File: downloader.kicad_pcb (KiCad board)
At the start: 2 copper layers, 30 x 15 mm, 16 parts, among them J1 USB_C_Receptacle_USB2.0, J2 Conn_01x06_Female, Q1 SS8050-G, Q2 SS8050-G, SW1 SW_Push, SW2 SW_Push, U1 AMS1117-3.3, U2 ch340k

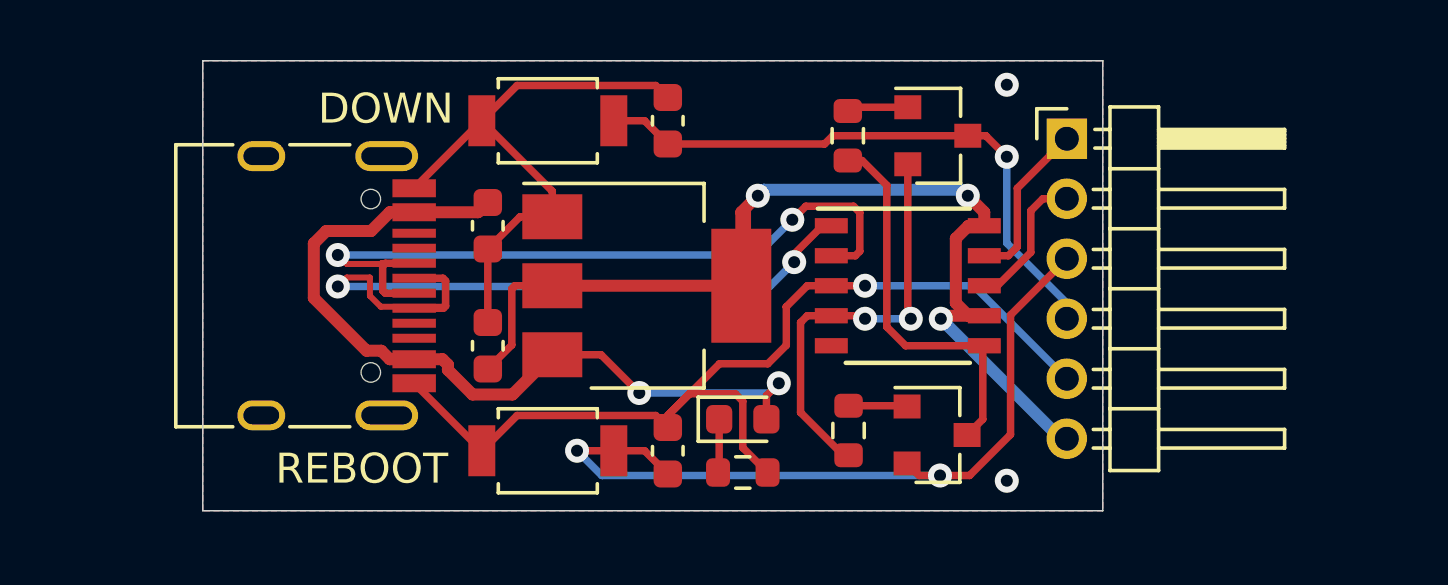
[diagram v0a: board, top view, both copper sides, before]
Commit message: version2.0
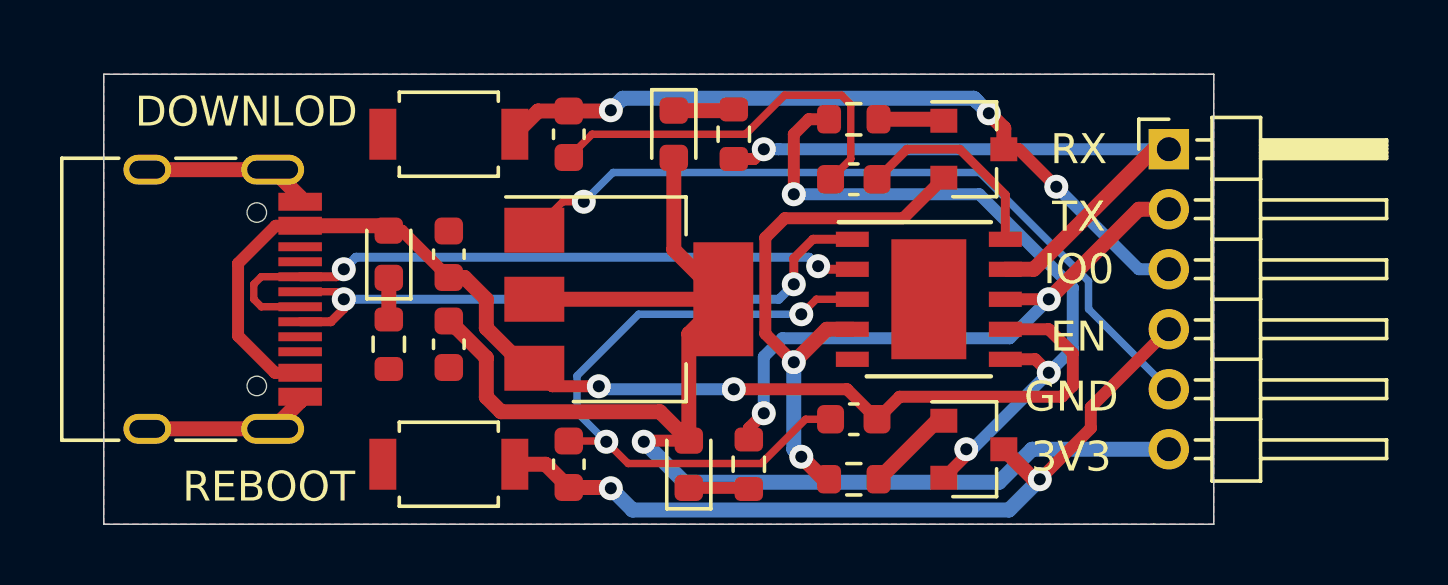
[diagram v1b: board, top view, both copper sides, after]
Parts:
- added C5: 0.1uf, Capacitor_SMD:C_0603_1608Metric, F.Cu at (112.2, 87.5)
- added C6: 0.1uf, Capacitor_SMD:C_0603_1608Metric, F.Cu at (112.2, 98.5)
- added D2: LED, Diode_SMD:D_0603_1608Metric, F.Cu at (115.7, 87.5)
- added D3: LED, Diode_SMD:D_0603_1608Metric, F.Cu at (116.2, 98.5)
- added R4: 10k, Resistor_SMD:R_0603_1608Metric, F.Cu at (121.7, 99.0)
- added R5: 10k, Resistor_SMD:R_0603_1608Metric, F.Cu at (121.7, 87.0)
- C2: value 0.1uf -> 10uf
- C3: value 10uf -> 0.1uf
- C4: value 0.1uf -> 0.1UF
- R1: value 470 -> 10k
- U2: footprint Package_SO:SSOP-10_3.9x4.9mm_P1.00mm -> my:ESSOP-10_3.9x4.9mm_P1.00mm
- moved C3 13.4 mm to (121.7, 89.0), turned to 0 degrees
- moved D1 13.0 mm to (106.2, 91.5), turned to 90 degrees
- moved R1 12.6 mm to (106.2, 94.5), turned to 270 degrees
- moved C2 10.4 mm to (108.2, 94.5), turned to 270 degrees
- moved C4 6.29 mm to (121.7, 97.0), turned to 0 degrees
- moved J1 3.83 mm to (99.2, 93.0)
- moved R2 3.80 mm to (117.7, 87.5)
- moved R3 3.51 mm to (118.2, 98.5), turned to 90 degrees
- moved J2 3.42 mm to (132.2, 88.0)
- moved SW1 3.33 mm to (108.2, 87.5)
- moved SW2 3.33 mm to (108.2, 98.5)
- moved C1 1.61 mm to (108.2, 91.5), turned to 90 degrees
- moved Q2 1.31 mm to (125.7, 98.0)
- moved Q1 1.28 mm to (125.7, 88.0)
- moved U2 0.83 mm to (124.2, 93.0)
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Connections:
- C1 pad 1: Net-(C1-Pad1) -> VCC
- C2 pad 1: /IO0 -> +3V3
- C3 pad 1: +3V3 -> GND
- C3 pad 2: GND -> Net-(C3-Pad2)
- C4 pad 1: /EN -> GND
- C4 pad 2: GND -> VCC
- D1 pad 2: Net-(C1-Pad1) -> VCC
- J1 pad A4: Net-(C1-Pad1) -> VCC
- J1 pad A5: Net-(J1-PadA5) -> (no net)
- J1 pad A8: Net-(J1-PadA8) -> (no net)
- J1 pad A9: Net-(C1-Pad1) -> VCC
- J1 pad B4: Net-(C1-Pad1) -> VCC
- J1 pad B5: Net-(J1-PadB5) -> (no net)
- J1 pad B8: Net-(J1-PadB8) -> (no net)
- J1 pad B9: Net-(C1-Pad1) -> VCC
- J2 pad 3: /EN -> /IO0
- J2 pad 4: /IO0 -> /EN
- Q2 pad 2: /EN -> /RTS
- Q2 pad 3: /RTS -> /EN
- R2 pad 1: Net-(Q1-Pad1) -> Net-(D2-Pad1)
- R2 pad 2: /RTS -> /RXD
- R3 pad 1: Net-(Q2-Pad1) -> Net-(D3-Pad1)
- R3 pad 2: /DTR -> /TXD
- U1 pad 3: Net-(C1-Pad1) -> VCC
- U2 pad 10: +3V3 -> Net-(C3-Pad2)
- U2 pad 5: Net-(U2-Pad5) -> (no net)
- U2 pad 7: +3V3 -> VCC
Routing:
- net VCC: track 0.00 -> 40.7 mm, vias 0 -> 2
- net Net-(C1-Pad1): track 27.7 -> 0.00 mm, vias 2 -> 0
- net GND: track 52.4 -> 72.4 mm, vias 2 -> 3
- net /RXD: track 5.51 -> 24.6 mm, vias 0 -> 1
- net /TXD: track 4.76 -> 20.0 mm, vias 0 -> 2
- net /RTS: track 13.1 -> 23.8 mm, vias 0 -> 3
- net +3V3: track 37.2 -> 47.3 mm, vias 3 -> 1
- net Net-(C3-Pad2): track 0.00 -> 6.80 mm
- net /IO0: track 20.1 -> 25.1 mm, vias 1 -> 3
- net /D+: track 26.8 -> 21.8 mm
- net /DTR: track 14.0 -> 18.2 mm
- net /D-: track 26.1 -> 22.6 mm
- net Net-(D3-Pad1): track 0.00 -> 2.02 mm
- net Net-(D2-Pad1): track 0.00 -> 2.02 mm
- net Net-(Q2-Pad1): track 2.14 -> 2.98 mm
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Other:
- board size 30 x 15 mm -> 37 x 15 mm
- board text added: "3V3"
- board text added: "DOWNLOD"
- board text added: "RX"
- board text added: "TX"
- board text removed: "+3.3V"
- board text removed: "DOWN"
- board text removed: "RXD"
- board text removed: "TXD"
